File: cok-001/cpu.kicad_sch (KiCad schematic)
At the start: 5 parts

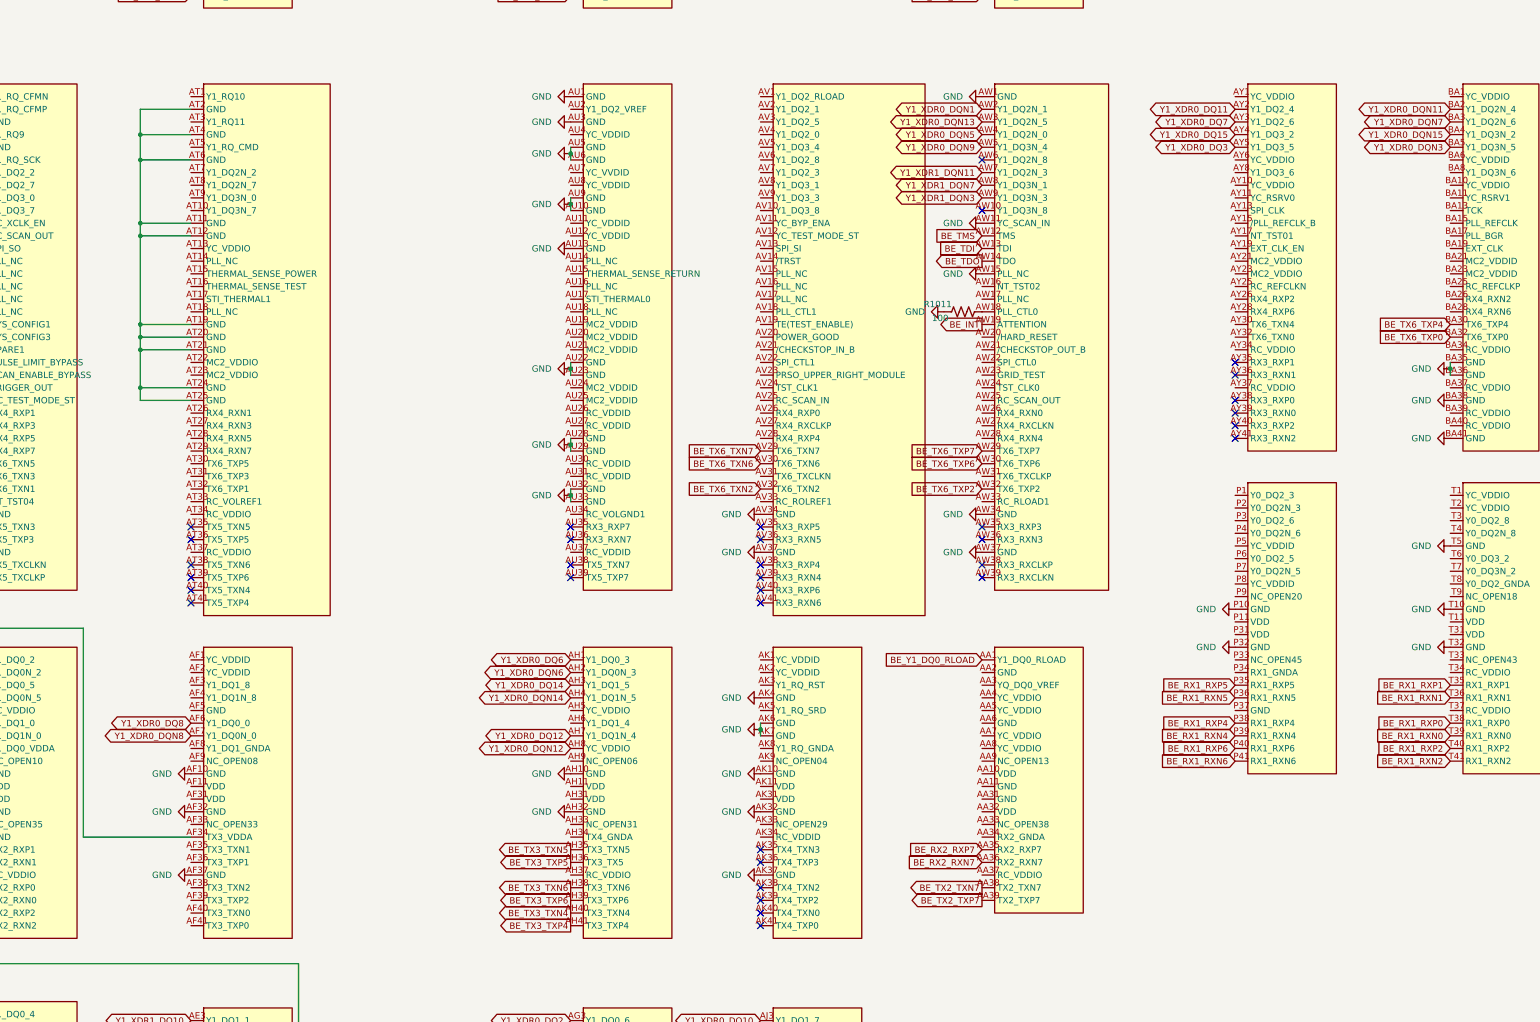
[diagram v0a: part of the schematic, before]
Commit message: rdy
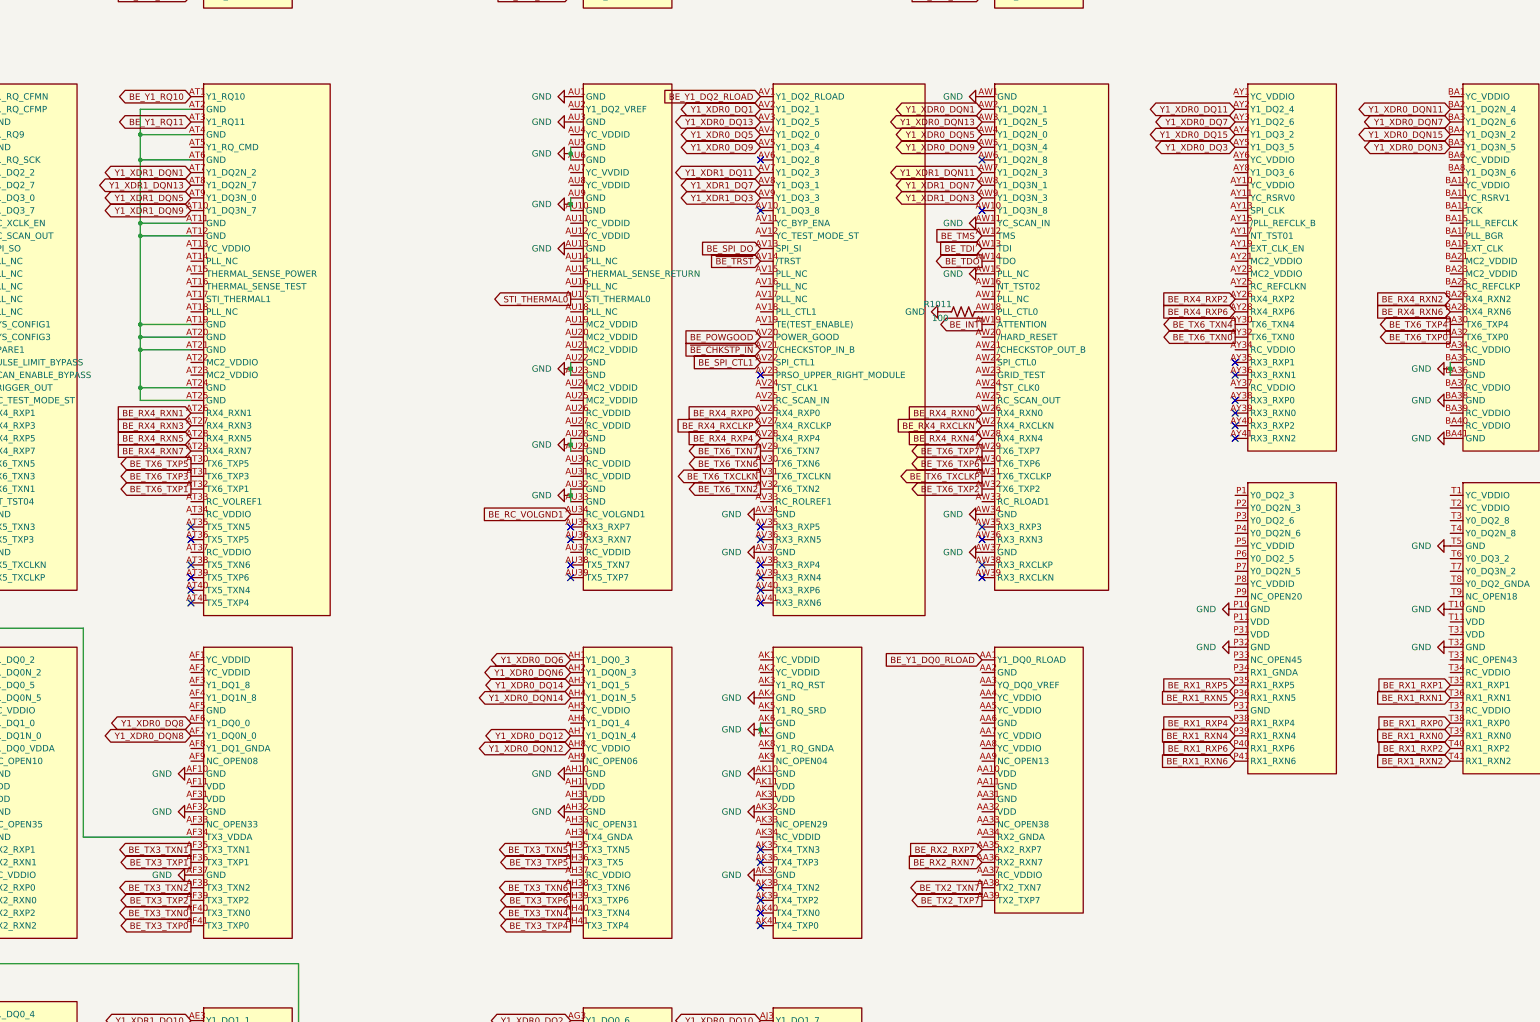
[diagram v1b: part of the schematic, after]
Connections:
- net Y1_XDR0_DQ1: now also U1001.AV2 (Y1_DQ2_1)
- net Y1_XDR0_DQ13: now also U1001.AV3 (Y1_DQ2_5)
- net Y1_XDR0_DQ5: now also U1001.AV4 (Y1_DQ2_0)
- net Y1_XDR0_DQ9: now also U1001.AV5 (Y1_DQ3_4)
- net Y1_XDR1_DQ11: now also U1001.AV7 (Y1_DQ2_3)
- net Y1_XDR1_DQ3: now also U1001.AV9 (Y1_DQ3_3)
- net Y1_XDR1_DQ7: now also U1001.AV8 (Y1_DQ3_1)
- net Y1_XDR1_DQN1: now also U1001.AT7 (Y1_DQ2N_2)
- net Y1_XDR1_DQN13: now also U1001.AT8 (Y1_DQ2N_7)
- net Y1_XDR1_DQN5: now also U1001.AT9 (Y1_DQ3N_0)
- net Y1_XDR1_DQN9: now also U1001.AT10 (Y1_DQ3N_7)
- net BE_RX4_RXN2: now reaches U1001.BA26 (RX4_RXN2)
- net BE_RX4_RXN6: now reaches U1001.BA28 (RX4_RXN6)
- net BE_Y1_RQ10: now reaches U1001.AT1 (Y1_RQ10)
- net BE_RX4_RXN1: now reaches U1001.AT26 (RX4_RXN1)
- net BE_RX4_RXN3: now reaches U1001.AT27 (RX4_RXN3)
- net BE_RX4_RXN5: now reaches U1001.AT28 (RX4_RXN5)
- net BE_RX4_RXN7: now reaches U1001.AT29 (RX4_RXN7)
- net BE_Y1_RQ11: now reaches U1001.AT3 (Y1_RQ11)
- net BE_TX6_TXP5: now reaches U1001.AT30 (TX6_TXP5)
- net BE_TX6_TXP3: now reaches U1001.AT31 (TX6_TXP3)
- net BE_TX6_TXP1: now reaches U1001.AT32 (TX6_TXP1)
- net BE_RX4_RXN0: now reaches U1001.AW26 (RX4_RXN0)
- net BE_RX4_RXCLKN: now reaches U1001.AW27 (RX4_RXCLKN)
- net BE_RX4_RXN4: now reaches U1001.AW28 (RX4_RXN4)
- net BE_TX6_TXCLKP: now reaches U1001.AW31 (TX6_TXCLKP)
- net BE_TX3_TXN1: now reaches U1001.AF35 (TX3_TXN1)
- net BE_TX3_TXP1: now reaches U1001.AF36 (TX3_TXP1)
- net BE_TX3_TXN2: now reaches U1001.AF38 (TX3_TXN2)
- net BE_TX3_TXP2: now reaches U1001.AF39 (TX3_TXP2)
- net BE_TX3_TXN0: now reaches U1001.AF40 (TX3_TXN0)
- net BE_TX3_TXP0: now reaches U1001.AF41 (TX3_TXP0)
- net BE_Y1_DQ2_RLOAD: now reaches U1001.AV1 (Y1_DQ2_RLOAD)
- net BE_SPI_DO: now reaches U1001.AV13 (SPI_SI)
- net ~{BE_TRST}: now reaches U1001.AV14 (/TRST)
- net BE_POWGOOD: now reaches U1001.AV20 (POWER_GOOD)
- net ~{BE_CHKSTP_IN}: now reaches U1001.AV21 (/CHECKSTOP_IN_B)
- net BE_SPI_CTL1: now reaches U1001.AV22 (SPI_CTL1)
- net BE_RX4_RXP0: now reaches U1001.AV26 (RX4_RXP0)
- net BE_RX4_RXCLKP: now reaches U1001.AV27 (RX4_RXCLKP)
- net BE_RX4_RXP4: now reaches U1001.AV28 (RX4_RXP4)
- net BE_TX6_TXCLKN: now reaches U1001.AV31 (TX6_TXCLKN)
- net BE_RX4_RXP2: now reaches U1001.AY26 (RX4_RXP2)
- net BE_RX4_RXP6: now reaches U1001.AY28 (RX4_RXP6)
- net BE_TX6_TXN4: now reaches U1001.AY30 (TX6_TXN4)
- net BE_TX6_TXN0: now reaches U1001.AY32 (TX6_TXN0)
- net STI_THERMAL0: now reaches U1001.AU17 (STI_THERMAL0)
- net BE_RC_VOLGND1: now reaches U1001.AU34 (RC_VOLGND1)
- no-connect marks 54 -> 57
